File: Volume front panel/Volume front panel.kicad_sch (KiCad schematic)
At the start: 29 parts, among them IC1 TLC5947DAPR, IC2 TPIC6B595DWR, J1 26-60-4023, J2 10129381-908001BLF, U1 PEC11R-4330F-S0012, U2 TSOP39238

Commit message: likely all done with v1, mainboard obsolete
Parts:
- removed C12: 0.1uf, Capacitor_SMD:C_1206_3216Metric, symbol Device:C_Small
- removed H1, H2, H3, H4: MountingHole, MountingHole:MountingHole_3.2mm_M3_ISO7380, symbol Mechanical:MountingHole
- removed IC2: TPIC6B595DWR, Samacsys:SOIC127P1030X265-20N, symbol Samacsys_kicad_sym:TPIC6B595DWR
- removed J1: 26-60-4023, Samacsys:26604023, symbol Samacsys:26-60-4023
- removed J2: 10129381-908001BLF, Samacsys:10129381908001BLF, symbol Samacsys:10129381-908001BLF
- removed R7: 10k, Resistor_SMD:R_1206_3216Metric, symbol Device:R_Small
- added C2, C3, C5: 0.01uf, Capacitor_SMD:C_1206_3216Metric, symbol Device:C_Small
- added J1, J2: BHR-06-VUA, Samacsys:SHDR6W64P254_2X3_1522X880X920P, symbol Samacsys:BHR-06-VUA
- added R1, R12, R2, R3, R4: 10k, Resistor_SMD:R_1206_3216Metric, symbol Device:R_Small
- added R11, R9: 4.7k, Resistor_SMD:R_1206_3216Metric, symbol Device:R_Small
- added U1: PEC11R-4330F-S0012, Samacsys:PEC11R4330FS0012, symbol Samacsys_kicad_sym:PEC11R-4330F-S0012
- renumbered C8 to C10, C10 to C11, C11 to C12, C2 to C4, C3 to C6, C4 to C7, C5 to C8, C6 to C9, R5 to R10, R6 to R13, R1 to R5, R2 to R6, R3 to R7, R4 to R8, U1 to U2, U2 to U3
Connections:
- net r_data is gone; now on net IR: A1.11 (D8)
- net shift_reg_clock is gone; now on an unnamed net: A1.8 (D5)
- net unmute is gone; now on an unnamed net: A1.10 (D7)
- net +5V: now also J1.1, J1.3, J1.5, J2.1, J2.2, R11.2, R2.2, R3.1, R9.2
- net GNDD: now also C2.1, C3.2, C5.2, J1.2, J1.4, J1.6, J2.3, J2.4, R12.1, U1.1 (COM), U1.C1 (COMMON)
- net blank: now also A1.21 (A2), R12.2; no longer A1.16 (D13)
- net data: now also A1.19 (A0); no longer A1.14 (D11)
- net sclk: now also A1.20 (A1); no longer A1.13 (D10)
- net xlat: now also A1.22 (A3); no longer A1.15 (D12)
- net at C7.1, U2.2 (NO): no longer A1.7 (D4)
- net IR: now reaches C10.1, U3.3 (OUT)
- net IR: no longer A1.12 (D9)
- net at C8.1, R8.2: no longer A1.6 (D3)
- net SDA: now reaches A1.23 (A4)
- net SDA: now also J2.6, R9.1
- net SCL: now reaches A1.24 (A5)
- net SCL: now also J2.5, R11.1
- net shift_reg_strobe: no longer names the net of A1.9 (D6)
- net shift_reg_strobe: now also C3.1, U1.2 (NO)
- new net: A1.6 (D3), C2.2, R1.2
- new net: R3.2, R4.1, U1.B1 (CHANNEL_B)
- new net: R1.1, R2.1, U1.A1 (CHANNEL_A)
- new net: A1.7 (D4), C5.1, R4.2

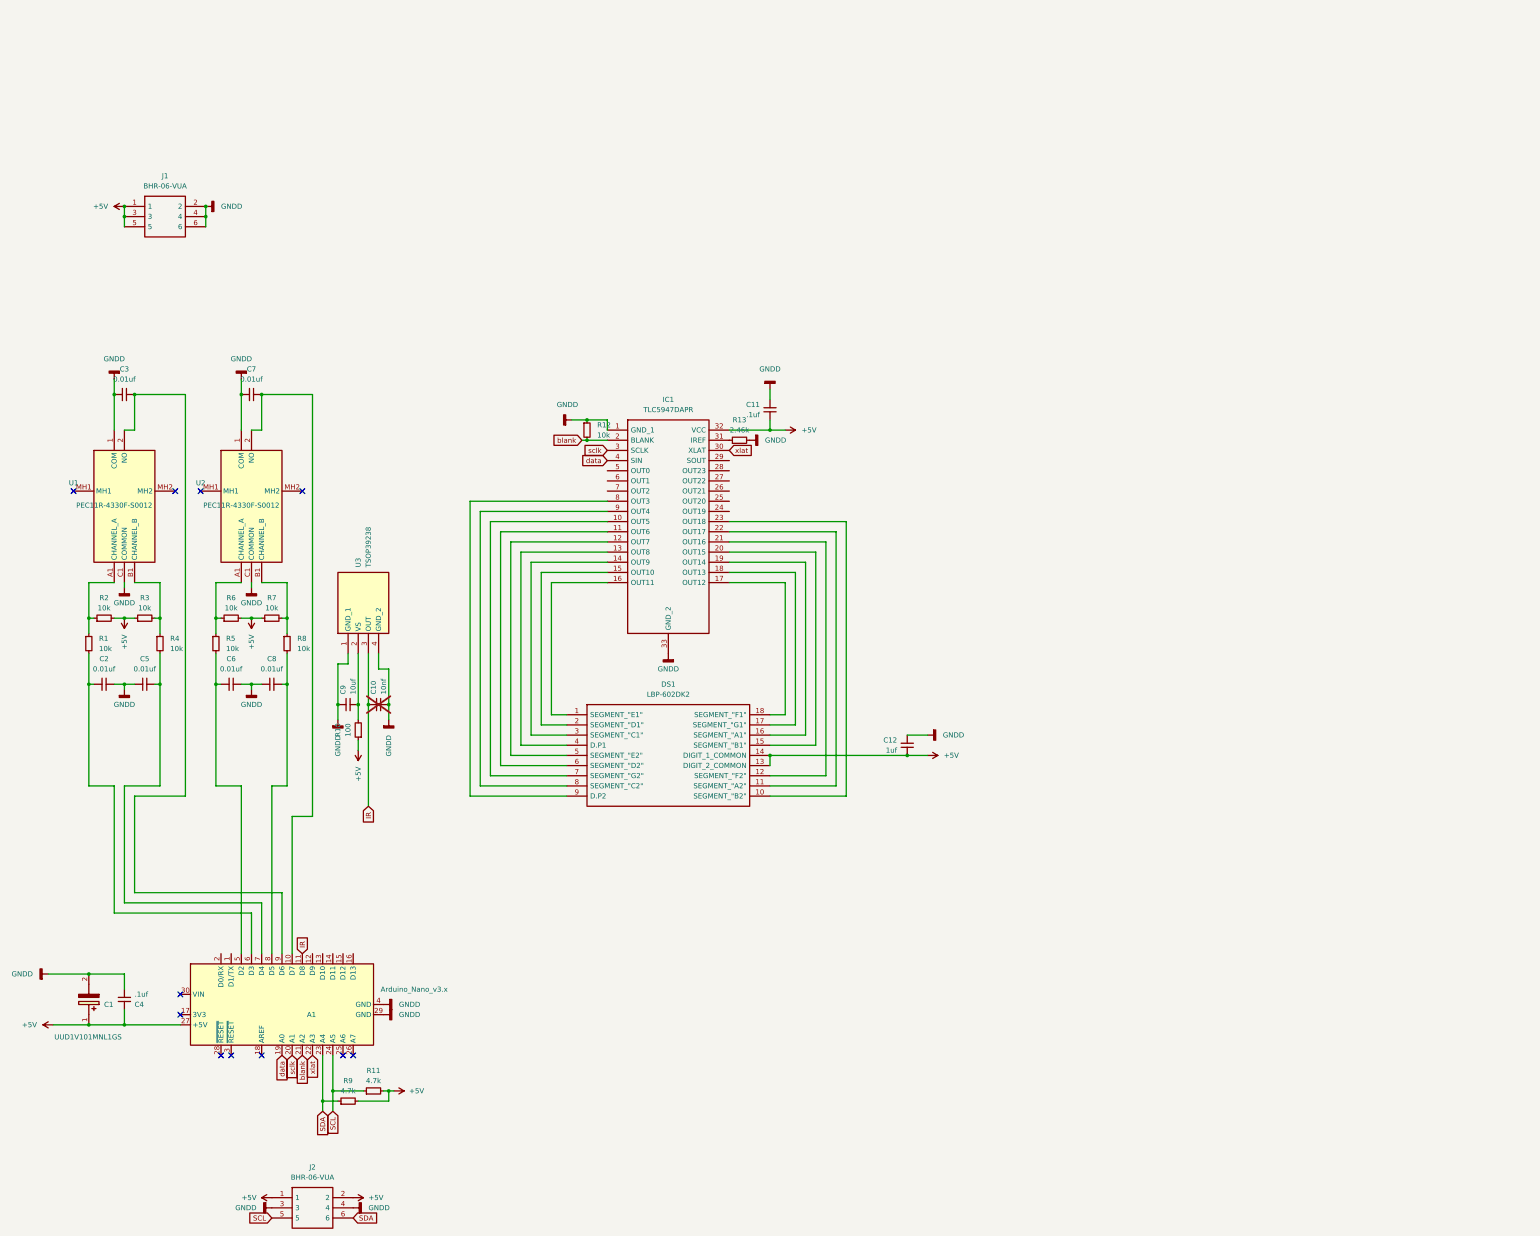
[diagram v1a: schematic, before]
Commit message: almost made 2040 raw
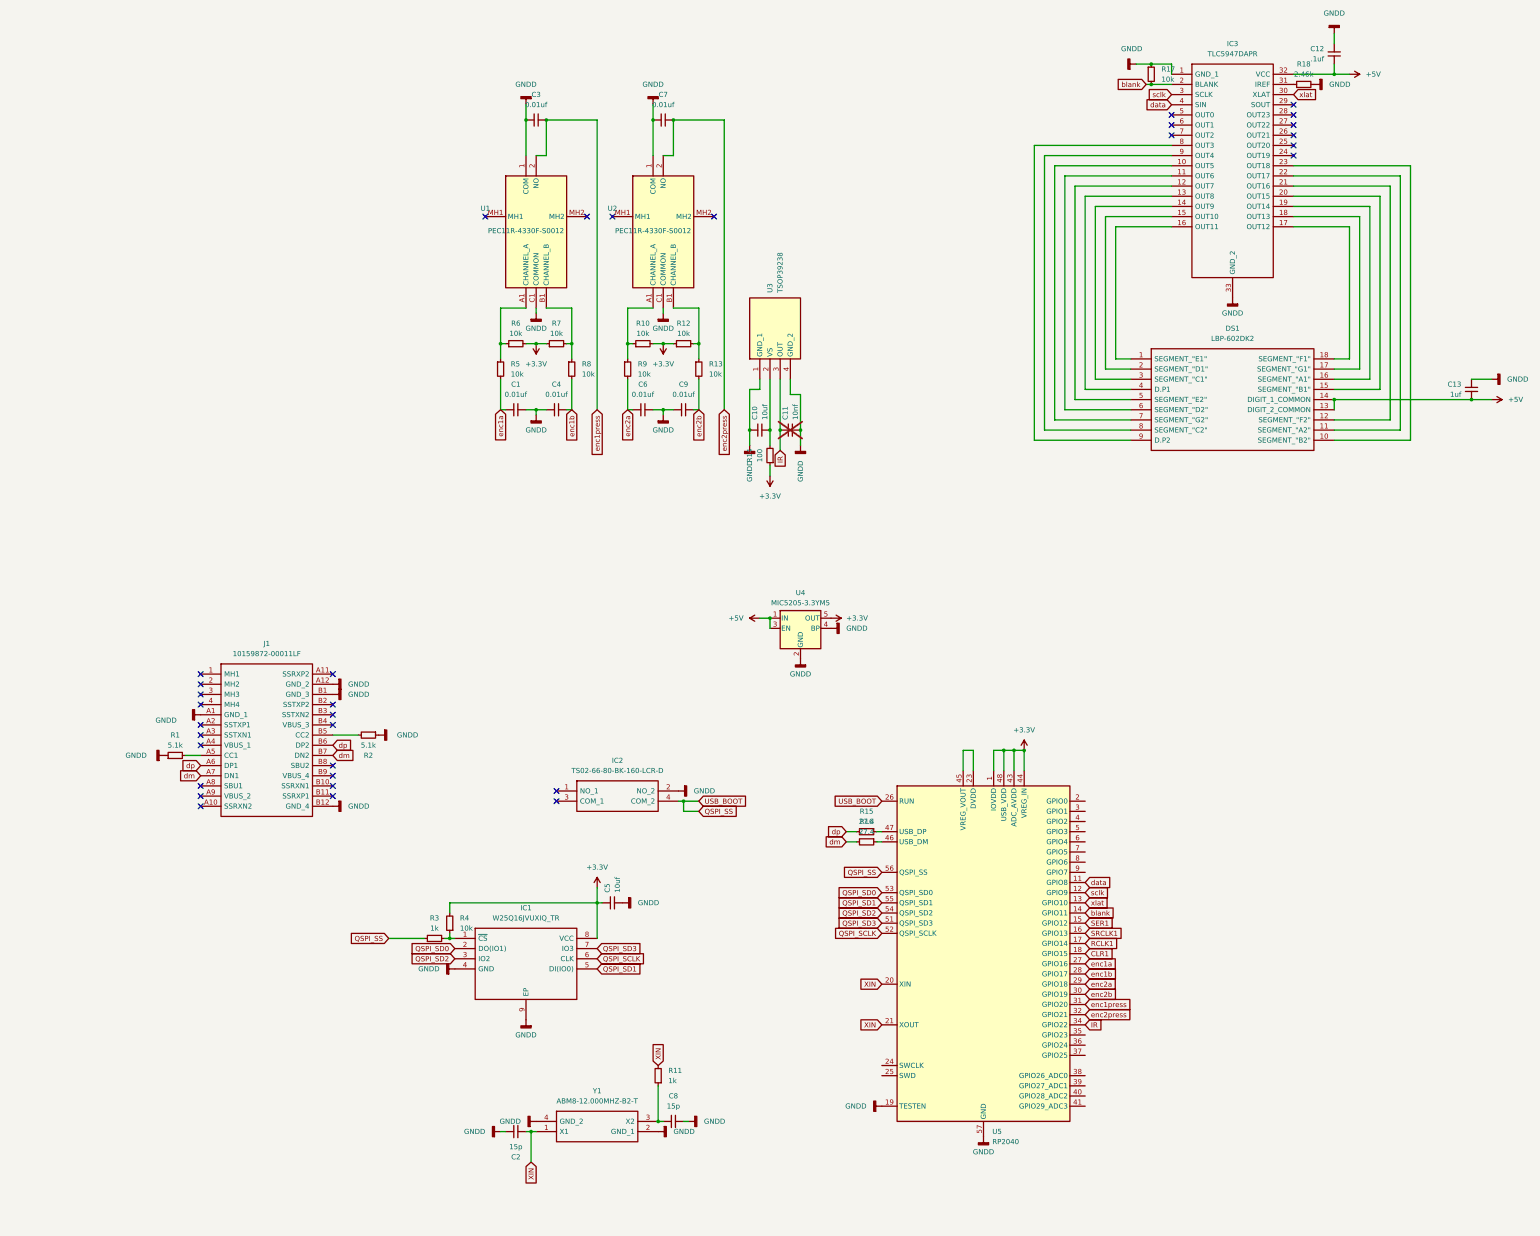
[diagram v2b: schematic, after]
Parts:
- removed A1: Arduino_Nano_v3.x, Module:Arduino_Nano, symbol MCU_Module:Arduino_Nano_v3.x
- removed C1: UUD1V101MNL1GS, Samacsys:CAPAE830X1050N, symbol Samacsys_kicad_sym:UUD1V101MNL1GS
- removed C4: .1uf, Capacitor_SMD:C_1206_3216Metric, symbol Device:C_Small
- removed J1, J2: BHR-06-VUA, Samacsys:SHDR6W64P254_2X3_1522X880X920P, symbol Samacsys:BHR-06-VUA
- removed R9: 4.7k, Resistor_SMD:R_1206_3216Metric, symbol Device:R_Small
- added C2, C8: 15p, Capacitor_SMD:C_1206_3216Metric, symbol Device:C_Small
- added C5: 10uf, Capacitor_SMD:C_1206_3216Metric, symbol Device:C_Small
- added IC1: W25Q16JVUXIQ_TR, Samacsys:SON50P300X200X60-9N, symbol Samacsys:W25Q16JVUXIQ_TR
- added IC2: TS02-66-80-BK-160-LCR-D, Samacsys:TS026680BK160LCRD, symbol Samacsys:TS02-66-80-BK-160-LCR-D
- added J1: 10159872-00011LF, Samacsys:1015987200011LF, symbol Samacsys:10159872-00011LF
- added R1, R2: 5.1k, Resistor_SMD:R_1206_3216Metric, symbol Device:R_Small
- added R15, R16: 27.4, Resistor_SMD:R_1206_3216Metric, symbol Device:R_Small
- added R3: 1k, Resistor_SMD:R_1206_3216Metric, symbol Device:R_Small
- added R4: 10k, Resistor_SMD:R_1206_3216Metric, symbol Device:R_Small
- added U4: MIC5205-3.3YM5, Package_TO_SOT_SMD:SOT-23-5, symbol Regulator_Linear:MIC5205-3.3YM5
- added U5: RP2040, Package_DFN_QFN:QFN-56-1EP_7x7mm_P0.4mm_EP3.2x3.2mm, symbol MCU_RaspberryPi:RP2040
- added Y1: ABM8-12.000MHZ-B2-T, Samacsys:ABM810000MHZ12D2W, symbol Samacsys:ABM8-12.000MHZ-B2-T
- R11: value 4.7k -> 1k
- renumbered C2 to C1, C9 to C10, C10 to C11, C11 to C12, C12 to C13, C5 to C4, C8 to C9, IC1 to IC3, R6 to R10, R7 to R12, R8 to R13, R10 to R14, R12 to R17, R13 to R18, R1 to R5, R2 to R6, R3 to R7, R4 to R8, R5 to R9
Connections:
- net +5V: now also U4.1 (IN), U4.3 (EN); no longer R10.2, R11.2, R12.1, R14.1, R6.2, R7.1
- net GNDD: now also C2.1, C5.2, C8.1, IC1.4 (GND), IC1.9 (EP), IC2.2 (NO_2), J1.A1 (GND_1), J1.A12 (GND_2), J1.B1 (GND_3), J1.B12 (GND_4), R1.1, R2.1, U4.2 (GND), U4.4 (BP), U5.19 (TESTEN), U5.57 (GND), Y1.2 (GND_1), Y1.4 (GND_2)
- net IR: now also U5.34 (GPIO22)
- net blank: now also U5.14 (GPIO11)
- net data: now also U5.11 (GPIO8)
- net sclk: now also U5.12 (GPIO9)
- net xlat: now also U5.13 (GPIO10)
- net enc1a: now reaches C1.2, R5.2
- net enc1a: now also U5.27 (GPIO16)
- net enc1press: now reaches C3.1, U1.2 (NO)
- net enc1press: now also U5.31 (GPIO20)
- net enc1b: now reaches C4.1, R8.2
- net enc1b: now also U5.28 (GPIO17)
- net enc2a: now reaches C6.2, R9.2
- net enc2a: now also U5.29 (GPIO18)
- net enc2press: now reaches C7.1, U2.2 (NO)
- net enc2press: now also U5.32 (GPIO21)
- net enc2b: now reaches C9.1, R13.2
- net enc2b: now also U5.30 (GPIO19)
- net SCL: no longer names the net of R11.1
- net SCL: now also C8.2, Y1.3 (X2)
- new net: IC1.1 (~{CS}), R3.2, R4.1
- new net: J1.A5 (CC1), R1.2
- new net: J1.B5 (CC2), R2.2
- new net: U5.23 (DVDD), U5.45 (VREG_VOUT), U5.50 (DVDD)
- new net: R16.1, U5.46 (USB_DM)
- new net: R15.1, U5.47 (USB_DP)
- new net +3.3V: C5.1, IC1.8 (VCC), R10.2, R12.1, R14.1, R4.2, R6.2, R7.1, U4.5 (OUT), U5.1 (IOVDD), U5.10 (IOVDD), U5.22 (IOVDD), U5.33 (IOVDD), U5.42 (IOVDD), U5.43 (ADC_AVDD), U5.44 (VREG_IN), U5.48 (USB_VDD), U5.49 (IOVDD)
- new net CLR1: U5.18 (GPIO15)
- new net QSPI_SCLK: IC1.6 (CLK), U5.52 (QSPI_SCLK)
- new net QSPI_SD0: IC1.2 (DO(IO1)), U5.53 (QSPI_SD0)
- new net QSPI_SD1: IC1.5 (DI(IO0)), U5.55 (QSPI_SD1)
- new net QSPI_SD2: IC1.3 (IO2), U5.54 (QSPI_SD2)
- new net QSPI_SD3: IC1.7 (IO3), U5.51 (QSPI_SD3)
- new net QSPI_SS: IC2.4 (COM_2), R3.1, U5.26 (RUN), U5.56 (QSPI_SS)
- new net RCLK1: U5.17 (GPIO14)
- new net SER1: U5.15 (GPIO12)
- new net SRCLK1: U5.16 (GPIO13)
- new net XIN: C2.2, R11.2, U5.20 (XIN), U5.21 (XOUT), Y1.1 (X1)
- new net dm: J1.A7 (DN1), J1.B7 (DN2), R16.2
- new net dp: J1.A6 (DP1), J1.B6 (DP2), R15.2
- no-connect marks 11 -> 33
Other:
- moved on the sheet: C1, C10, C11, C12, C13, C3, C4, C6, C7, C9, DS1, IC3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

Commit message: pico front panel so easy
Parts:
- removed C2, C8: 15p, Capacitor_SMD:C_1206_3216Metric, symbol Device:C_Small
- removed C5: 10uf, Capacitor_SMD:C_1206_3216Metric, symbol Device:C_Small
- removed IC1: W25Q16JVUXIQ_TR, Samacsys:SON50P300X200X60-9N, symbol Samacsys:W25Q16JVUXIQ_TR
- removed IC2: TS02-66-80-BK-160-LCR-D, Samacsys:TS026680BK160LCRD, symbol Samacsys:TS02-66-80-BK-160-LCR-D
- removed J1: 10159872-00011LF, Samacsys:1015987200011LF, symbol Samacsys:10159872-00011LF
- removed R1, R2: 5.1k, Resistor_SMD:R_1206_3216Metric, symbol Device:R_Small
- removed R11, R3: 1k, Resistor_SMD:R_1206_3216Metric, symbol Device:R_Small
- removed R15, R16: 27.4, Resistor_SMD:R_1206_3216Metric, symbol Device:R_Small
- removed R4: 10k, Resistor_SMD:R_1206_3216Metric, symbol Device:R_Small
- removed U4: MIC5205-3.3YM5, Package_TO_SOT_SMD:SOT-23-5, symbol Regulator_Linear:MIC5205-3.3YM5
- removed U5: RP2040, Package_DFN_QFN:QFN-56-1EP_7x7mm_P0.4mm_EP3.2x3.2mm, symbol MCU_RaspberryPi:RP2040
- removed Y1: ABM8-12.000MHZ-B2-T, Samacsys:ABM810000MHZ12D2W, symbol Samacsys:ABM8-12.000MHZ-B2-T
- added J1: TFM-105-01-F-D, Samacsys:TFM-105-XX-YYY-D, symbol Samacsys:TFM-105-01-F-D
- added J2: 26-60-4023, Samacsys:26604023, symbol Samacsys:26-60-4023
- added PS1: TMPW_5-105, Samacsys:TMPW5112, symbol Samacsys_kicad_sym:TMPW_5-105
- added U4: Pico, MCU_RaspberryPi_and_Boards:RPi_Pico_SMD_TH, symbol MCU_RaspberryPi_and_Boards:Pico
- renumbered C13 to C10, C3 to C2, C4 to C3, C6 to C4, C7 to C5, C9 to C6, C10 to C7, C11 to C8, C12 to C9, IC3 to IC1, R5 to R1, R17 to R10, R18 to R11, R6 to R2, R7 to R3, R8 to R4, R9 to R5, R10 to R6, R12 to R7, R13 to R8, R14 to R9
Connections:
- net +3.3V: now also J1.8, U4.36 (3V3)
- net +5V: now also J1.1, J1.2, J1.4, PS1.2 (+VOUT), U4.39 (VSYS)
- net GNDD: now also J1.3, J1.5, J1.6, PS1.3 (-VOUT), U4.13 (GND), U4.18 (GND), U4.23 (GND), U4.28 (GND), U4.3 (GND), U4.33 (AGND), U4.38 (GND), U4.42 (GND), U4.8 (GND)
- net IR: now also U4.20 (GPIO15)
- net RCLK1: now also J1.7, U4.7 (GPIO5)
- net SER1: now also J1.10, U4.10 (GPIO7)
- net SRCLK1: now also J1.9, U4.9 (GPIO6)
- net blank: now also U4.12 (GPIO9)
- net data: now also U4.14 (GPIO10)
- net enc1a: now also U4.1 (GPIO0)
- net enc1b: now also U4.2 (GPIO1)
- net enc1press: now also U4.4 (GPIO2)
- net enc2a: now also U4.17 (GPIO13)
- net enc2b: now also U4.19 (GPIO14)
- net enc2press: now also U4.16 (GPIO12)
- net sclk: now also U4.15 (GPIO11)
- net xlat: now also U4.11 (GPIO8)
- new net: J2.2, PS1.4 (AC_IN_(L))
- new net: J2.1, PS1.5 (AC_IN_(N))
- no-connect marks 33 -> 15
